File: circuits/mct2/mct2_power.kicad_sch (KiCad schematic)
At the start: 226 parts, among them J3 USB_C_Receptacle, J4 USB_C_Receptacle, U4 TPD4EUSB30, U5 TPD4EUSB30, U6 TPD4EUSB30, U7 TPD4EUSB30, U9 TPD6S300A

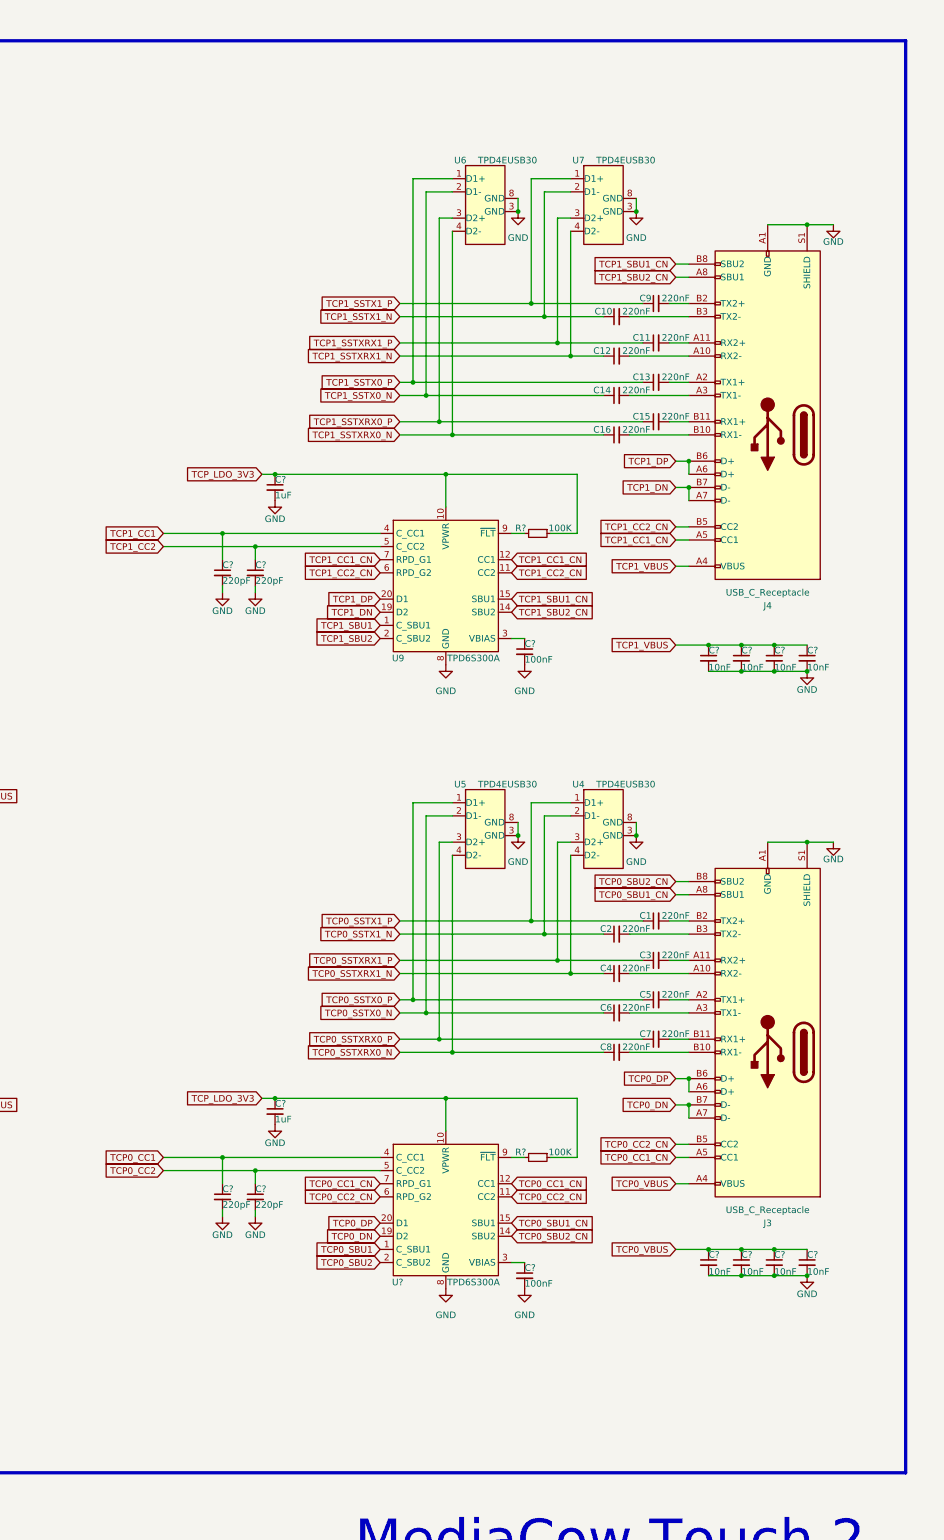
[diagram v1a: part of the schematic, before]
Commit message: Aug 28, 2024
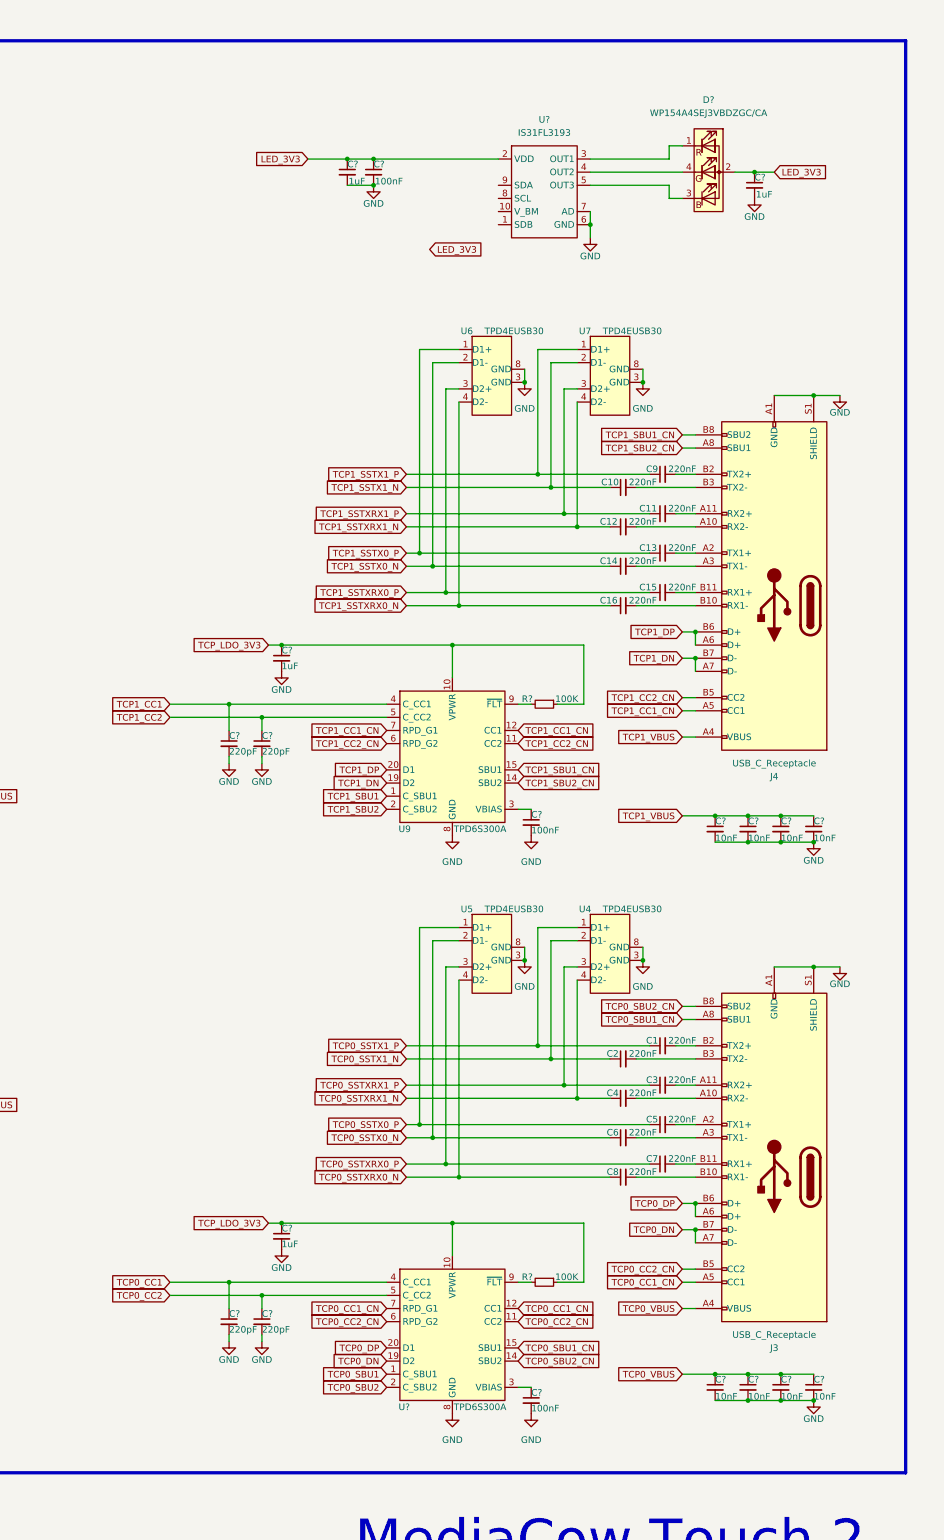
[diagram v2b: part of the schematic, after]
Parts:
- added C? (x2): 1uF, symbol Device:C_Small
- added C?: 100nF, symbol Device:C_Small
- added D?: WP154A4SEJ3VBDZGC/CA, Connector_PinSocket_1.27mm:PinSocket_1x04_P1.27mm_Vertical, symbol Device:LED_RABG
- added U?: IS31FL3193, Package_DFN_QFN:DFN-10-1EP_3x3mm_P0.5mm_EP1.75x2.7mm, symbol mediacow:IS31FL3193
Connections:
- net GND: now also C?.2, C?.2, C?.2, U?.6 (GND), U?.7 (AD)
- new net: D?.1 (RK), U?.3 (OUT1)
- new net: D?.3 (BK), U?.5 (OUT3)
- new net: D?.4 (GK), U?.4 (OUT2)
- new net LED_3V3: C?.1, C?.1, C?.1, D?.2 (A), U?.2 (VDD)
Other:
- moved on the sheet: C1, C10, C11, C12, C13, C14, C15, C16, C2, C3, C4, C5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
